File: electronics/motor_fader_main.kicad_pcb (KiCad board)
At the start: 2 copper layers, 59 x 17 mm, 32 parts, among them J1 Conn_01x05, J2 Program, J3 Conn_01x05, J4 Conn_01x04_MountingPin, J5 Conn_01x04_MountingPin, U1 ATtiny1616-M, U2 DRV8837

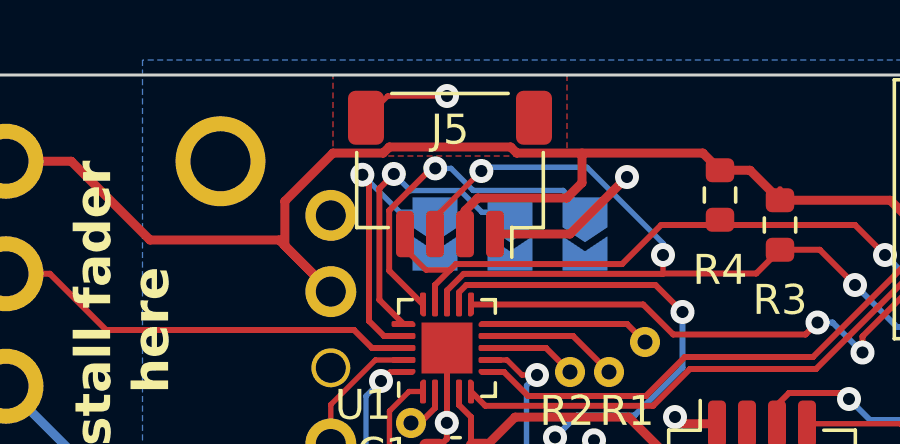
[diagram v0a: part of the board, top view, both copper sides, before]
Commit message: 3d model and update links in readme
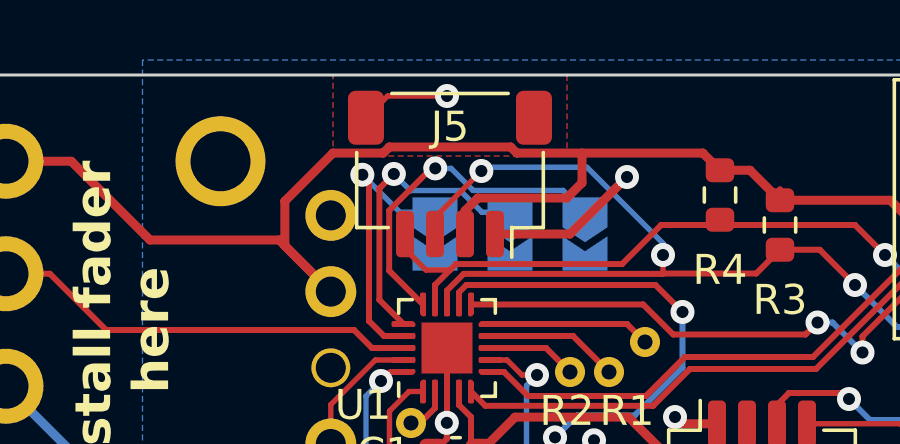
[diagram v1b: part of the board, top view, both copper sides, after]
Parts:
- J4, J5: footprint Connector_JST:JST_SH_SM04B-SRSS-TB_1x04-1MP_P1.00mm_Horizontal -> modified:JST_SH_SM04B-SRSS-TB_1x04-1MP_P1.00mm_Horizontal
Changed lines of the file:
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@@
 		)
 	)
-	(footprint "Connector_JST:JST_SH_SM04B-SRSS-TB_1x04-1MP_P1.00mm_Horizontal"
+	(footprint "modified:JST_SH_SM04B-SRSS-TB_1x04-1MP_P1.00mm_Horizontal"
 		(layer "F.Cu")
 		(at 81.4 55.125)
@@
 			)
 		)
-		(property "Footprint" "Connector_JST:JST_SH_SM04B-SRSS-TB_1x04-1MP_P1.00mm_Horizontal"
+		(property "Footprint" "modified:JST_SH_SM04B-SRSS-TB_1x04-1MP_P1.00mm_Horizontal"
 			(at 0 0 0)
 			(unlocked yes)
@@
 		)
 		(model "${KICAD8_3DMODEL_DIR}/Connector_JST.3dshapes/JST_SH_SM04B-SRSS-TB_1x04-1MP_P1.00mm_Horizontal.wrl"
+			(hide yes)
 			(offset
 				(xyz 0 0 0)
@@
 			(rotate
 				(xyz 0 0 0)
+			)
+		)
+		(model "${KIPRJMOD}/lib/misc.3dmodels/SM04B-SRSS-TB.STEP"
+			(offset
+				(xyz 0 1.3 -0.3)
+			)
+			(scale
+				(xyz 1 1 1)
+			)
+			(rotate
+				(xyz -90 0 0)
 			)
 		)
@@
 		)
 	)
-	(footprint "Connector_JST:JST_SH_SM04B-SRSS-TB_1x04-1MP_P1.00mm_Horizontal"
+	(footprint "modified:JST_SH_SM04B-SRSS-TB_1x04-1MP_P1.00mm_Horizontal"
 		(layer "F.Cu")
 		(at 71 44.8 180)
@@
 		(tags "connector JST SH horizontal")
 		(property "Reference" "J5"
-			(at 0 1.475 0)
+			(at 0 1.575 180)
 			(layer "F.SilkS")
 			(effects
@@
 		)
 		(property "Value" "Conn_01x04_MountingPin"
-			(at 0 3.98 0)
-			(layer "F.Fab")
-			(effects
-				(font
-					(size 1 1)
-					(thickness 0.15)
-				)
-			)
-		)
-		(property "Footprint" "Connector_JST:JST_SH_SM04B-SRSS-TB_1x04-1MP_P1.00mm_Horizontal"
+			(at 0 3.98 180)
+			(layer "F.Fab")
+			(effects
+				(font
+					(size 1 1)
+					(thickness 0.15)
+				)
+			)
+		)
+		(property "Footprint" "modified:JST_SH_SM04B-SRSS-TB_1x04-1MP_P1.00mm_Horizontal"
 			(at 0 0 180)
 			(unlocked yes)
@@
 		)
 		(fp_text user "${REFERENCE}"
-			(at 0 0 0)
+			(at 0 0 180)
 			(layer "F.Fab")
 			(effects
@@
 		)
 		(model "${KICAD8_3DMODEL_DIR}/Connector_JST.3dshapes/JST_SH_SM04B-SRSS-TB_1x04-1MP_P1.00mm_Horizontal.wrl"
+			(hide yes)
 			(offset
 				(xyz 0 0 0)
@@
 			)
 		)
+		(model "${KIPRJMOD}/lib/misc.3dmodels/SM04B-SRSS-TB.STEP"
+			(offset
+				(xyz 0 1.3 -0.3)
+			)
+			(scale
+				(xyz 1 1 1)
+			)
+			(rotate
+				(xyz -90 0 0)
+			)
+		)
